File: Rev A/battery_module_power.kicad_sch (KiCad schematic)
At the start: 17 parts, among them Q1 IRLZ44N, Q2 BC337, Q4 BC337, Q5 BC327

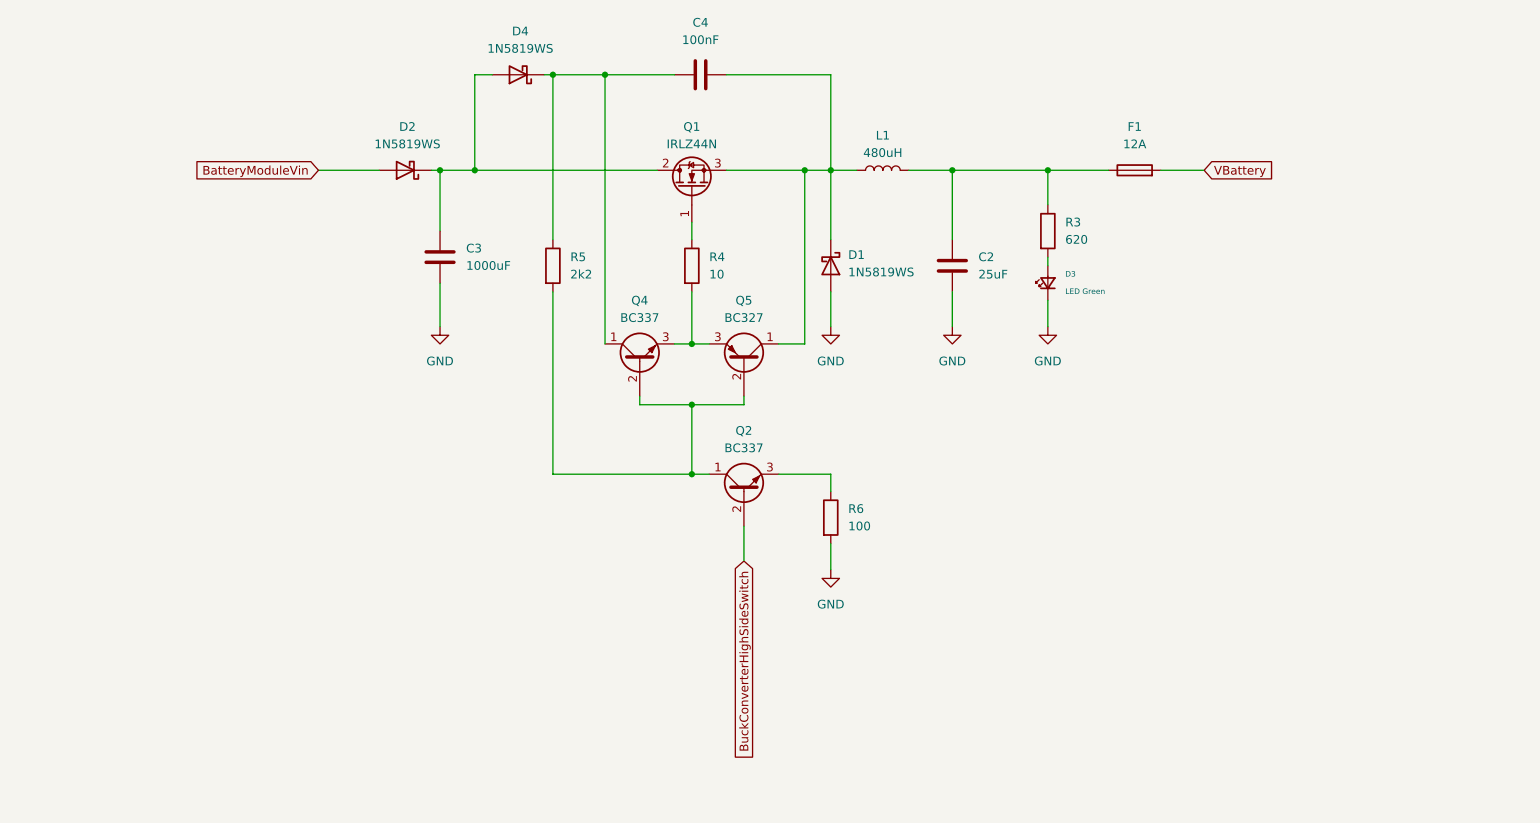
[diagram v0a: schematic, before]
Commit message: Updated PCB and Schematics
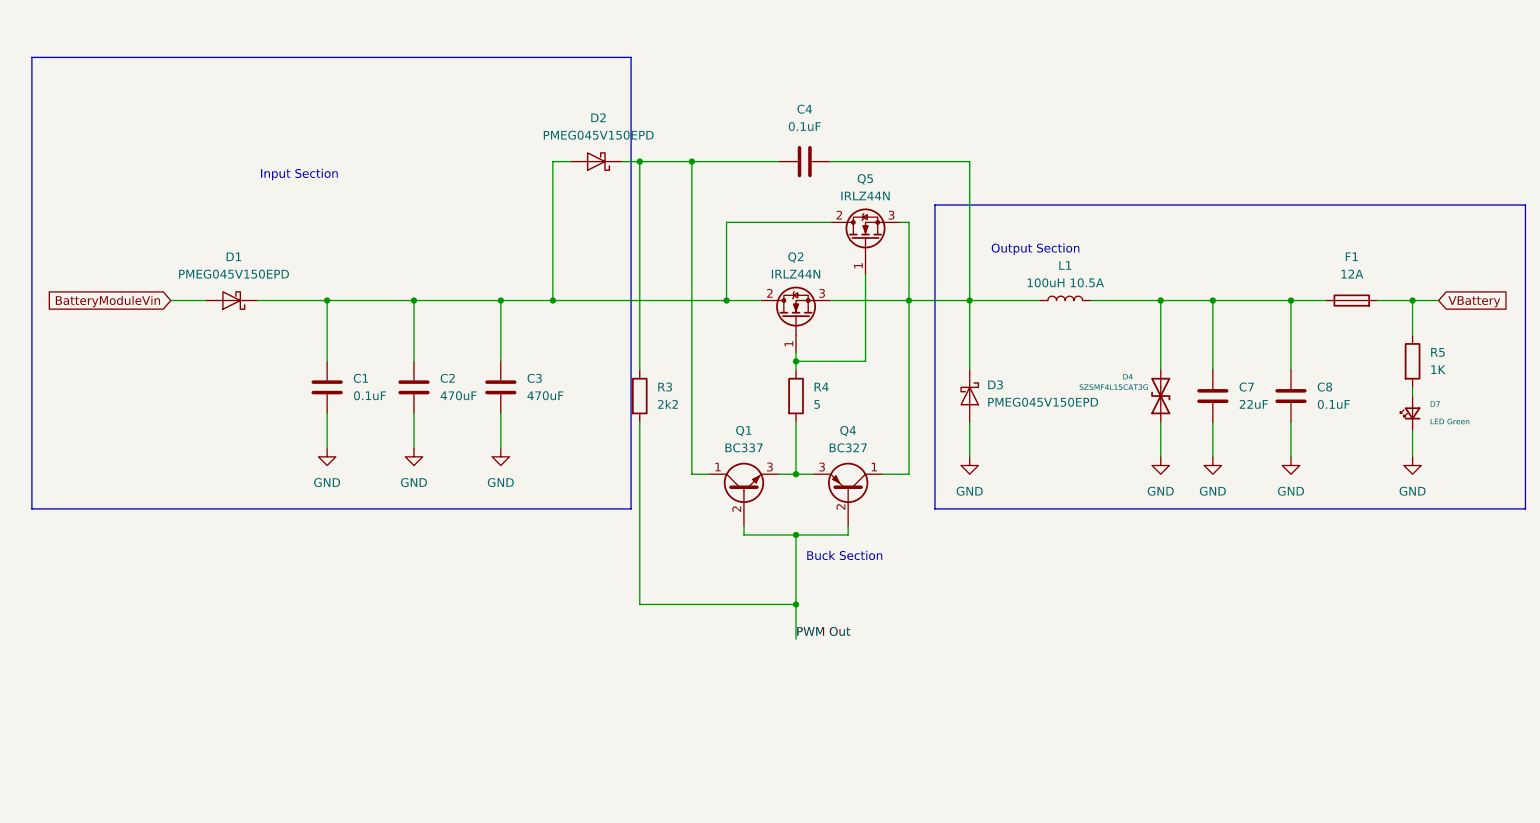
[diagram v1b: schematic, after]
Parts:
- removed D1, D2, D4: 1N5819WS, Diode_SMD:D_SOD-323, symbol Diode:1N5819WS
- removed D3: LED Green, LED_SMD:LED_0805_2012Metric, symbol Device:LED_Small
- removed Q1: IRLZ44N, Package_TO_SOT_THT:TO-220-3_Vertical, symbol Transistor_FET:IRLZ44N
- removed Q2, Q4: BC337, Package_TO_SOT_THT:TO-92_Inline, symbol Transistor_BJT:BC337
- removed Q5: BC327, Package_TO_SOT_THT:TO-92_Inline, symbol Transistor_BJT:BC327
- removed R6: 100, symbol Device:R
- added C1, C8: 0.1uF, Capacitor_SMD:C_0805_2012Metric, symbol Device:C
- added C7: 22uF, Capacitor_SMD:C_0805_2012Metric_Pad1.18x1.45mm_HandSolder, symbol Device:C
- added D1, D2, D3: PMEG045V150EPD, Package_TO_SOT_SMD:Nexperia_CFP15_SOT-1289, symbol Diode:PMEG045V150EPD
- added D4: SZSMF4L15CAT3G, Diode_SMD:D_SOD-123F, symbol Device:D_TVS
- added D7: LED Green, LED_SMD:LED_0805_2012Metric, symbol Device:LED_Small
- added Q1: BC337, Package_TO_SOT_THT:TO-92_Inline, symbol Transistor_BJT:BC337
- added Q2, Q5: IRLZ44N, Package_TO_SOT_THT:TO-220-3_Vertical, symbol Transistor_FET:IRLZ44N
- added Q4: BC327, Package_TO_SOT_THT:TO-92_Inline, symbol Transistor_BJT:BC327
- C2: value 25uF -> 470uF; footprint (none) -> Capacitor_SMD:C_0805_2012Metric_Pad1.18x1.45mm_HandSolder
- C3: value 1000uF -> 470uF; footprint (none) -> Capacitor_SMD:C_0805_2012Metric_Pad1.18x1.45mm_HandSolder
- C4: value 100nF -> 0.1uF; footprint (none) -> Capacitor_SMD:C_0805_2012Metric
- F1: footprint (none) -> Fuse:Fuse_0805_2012Metric_Pad1.15x1.40mm_HandSolder
- L1: value 480uH -> 100uH 10.5A; footprint (none) -> Inductor_SMD:L_0805_2012Metric
- R3: value 620 -> 2k2; footprint (none) -> Resistor_SMD:R_0805_2012Metric
- R4: value 10 -> 5; footprint (none) -> Resistor_SMD:R_0805_2012Metric
- R5: value 2k2 -> 1K; footprint (none) -> Resistor_SMD:R_0805_2012Metric
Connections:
- net BatteryModuleVin: now also D1.1 (A), D1.2 (A)
- net GND: now also C1.2, C7.2, C8.2, D3.1 (A), D3.2 (A), D4.1 (A1), D7.1 (K)
- net VBattery: now also R5.1
- net at R5.2: now also D7.2 (A)
- net at F1.1, L1.2: now also C7.1, C8.1, D4.2 (A2); no longer C2.1, R3.1
- net PWM Out: now reaches R3.2
- net PWM Out: now also Q1.2 (B), Q4.2 (B)
- net at C4.1: now also R3.1, D2.3 (K), Q1.1 (C); no longer R5.1
- net at C3.1: now also C2.1, C1.1, D1.3 (K), D2.1 (A), D2.2 (A), Q2.2 (D), Q5.2 (D)
- net at R4.2: now also Q1.3 (E), Q4.3 (E)
- net at C4.2, L1.1: now also D3.3 (K), Q2.3 (S), Q4.1 (C), Q5.3 (S)
- net at R4.1: now also Q2.1 (G), Q5.1 (G)
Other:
- note added: "Buck Section"
- note added: "Input Section"
- note added: "Output Section"
